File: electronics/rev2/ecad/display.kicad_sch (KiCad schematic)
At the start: 36 parts, among them Q1 2N7002, Q12 2N7002, Q14 2N7002, Q15 2N7002, Q16 2N7002, Q2 2N7002, Q3 2N7002, Q4 2N7002, U4 CC56-12SURKWA, U5 MCP23008-xSO

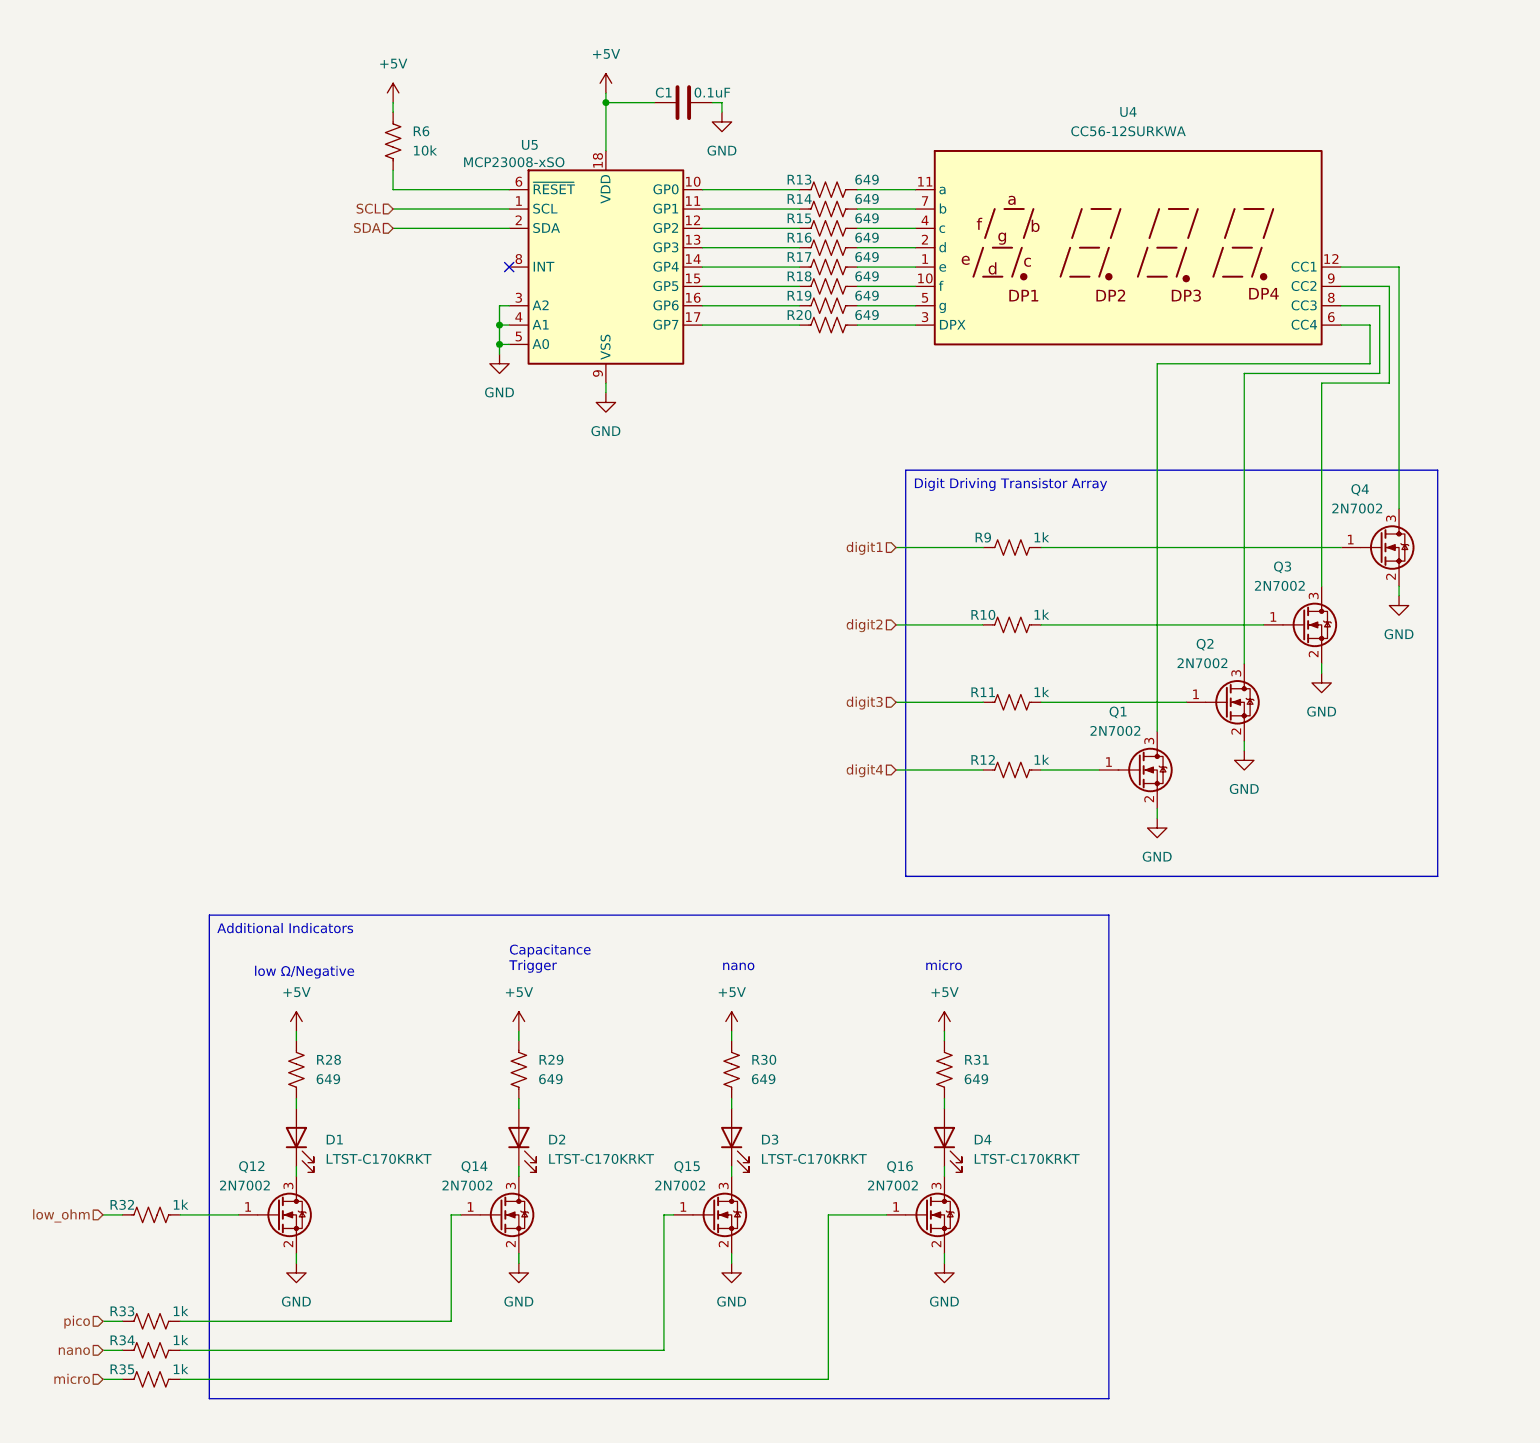
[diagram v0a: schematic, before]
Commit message: ordered some stuff
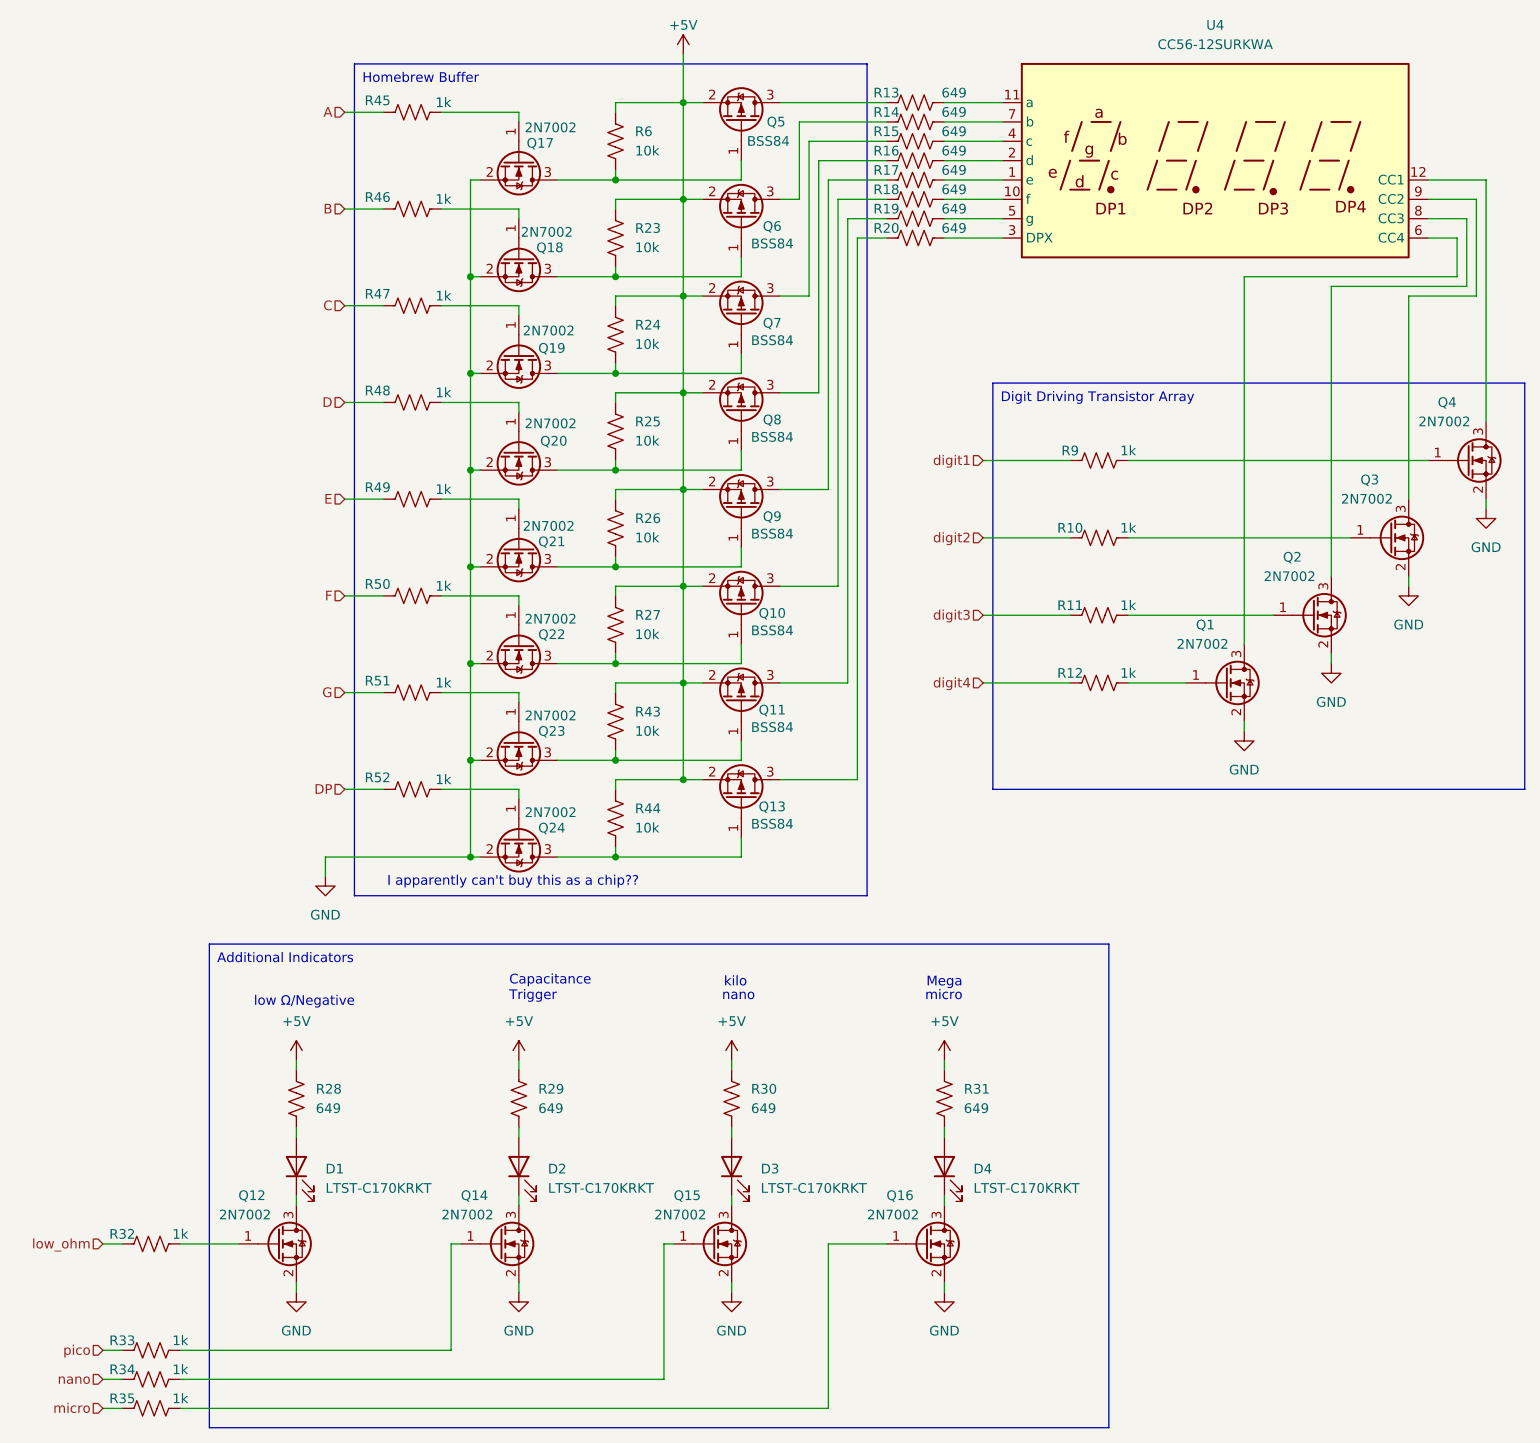
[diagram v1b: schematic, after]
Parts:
- removed C1: 0.1uF, Capacitor_SMD:C_0805_2012Metric, symbol Device:C
- removed U5: MCP23008-xSO, Package_SO:SOIC-18W_7.5x11.6mm_P1.27mm, symbol Interface_Expansion:MCP23008-xSO
- added Q10, Q11, Q13, Q5, Q6, Q7, Q8, Q9: BSS84, Package_TO_SOT_SMD:SOT-23, symbol Transistor_FET:BSS84
- added Q17, Q18, Q19, Q20, Q21, Q22, Q23, Q24: 2N7002, Package_TO_SOT_SMD:SOT-23, symbol Transistor_FET:2N7002
- added R23, R24, R25, R26, R27, R43, R44: 10k, Resistor_SMD:R_0805_2012Metric_Pad1.20x1.40mm_HandSolder, symbol Device:R_US
- added R45, R46, R47, R48, R49, R50, R51, R52: 1k, Resistor_SMD:R_0805_2012Metric_Pad1.20x1.40mm_HandSolder, symbol Device:R_US
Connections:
- net +5V: now also Q10.2 (S), Q11.2 (S), Q13.2 (S), Q5.2 (S), Q6.2 (S), Q7.2 (S), Q8.2 (S), Q9.2 (S), R23.1, R24.1, R25.1, R26.1, R27.1, R43.1, R44.1
- net GND: now also Q17.2 (S), Q18.2 (S), Q19.2 (S), Q20.2 (S), Q21.2 (S), Q22.2 (S), Q23.2 (S), Q24.2 (S)
- net at R17.1: now also Q9.3 (D)
- net at R13.1: now also Q5.3 (D)
- net at R14.1: now also Q6.3 (D)
- net at R15.1: now also Q7.3 (D)
- net at R16.1: now also Q8.3 (D)
- net at R18.1: now also Q10.3 (D)
- net at R19.1: now also Q11.3 (D)
- net at R20.1: now also Q13.3 (D)
- net at R6.2: now also Q17.3 (D), Q5.1 (G)
- new net: Q13.1 (G), Q24.3 (D), R44.2
- new net: Q11.1 (G), Q23.3 (D), R43.2
- new net: Q19.3 (D), Q7.1 (G), R24.2
- new net: Q21.3 (D), Q9.1 (G), R26.2
- new net: Q24.1 (G), R52.2
- new net: Q17.1 (G), R45.2
- new net: Q18.1 (G), R46.2
- new net: Q18.3 (D), Q6.1 (G), R23.2
- new net: Q22.1 (G), R50.2
- new net: Q10.1 (G), Q22.3 (D), R27.2
- new net: Q21.1 (G), R49.2
- new net: Q20.3 (D), Q8.1 (G), R25.2
- new net: Q19.1 (G), R47.2
- new net: Q20.1 (G), R48.2
- new net: Q23.1 (G), R51.2
- new net A: R45.1
- new net B: R46.1
- new net C: R47.1
- new net D: R48.1
- new net DP: R52.1
- new net E: R49.1
- new net F: R50.1
- new net G: R51.1
- no-connect marks 1 -> 0
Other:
- note added: "I apparently can't buy this as a chip??"
- note added: "Mega"
- note added: "kilo"
- moved on the sheet: D1, D2, D3, D4, Q1, Q12, Q14, Q15, Q16, Q2, Q3, Q4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
